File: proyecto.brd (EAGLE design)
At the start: 95.8 x 48.2 mm, 51 parts, among them IC1 ADE9153AACPZ, J1 796638-3, K1 PR28-3V-360-1A-E, Q1 12.288M, Q2 BSS123, U1 ESP32-PICO-MINI-02-N8R2ESP32-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

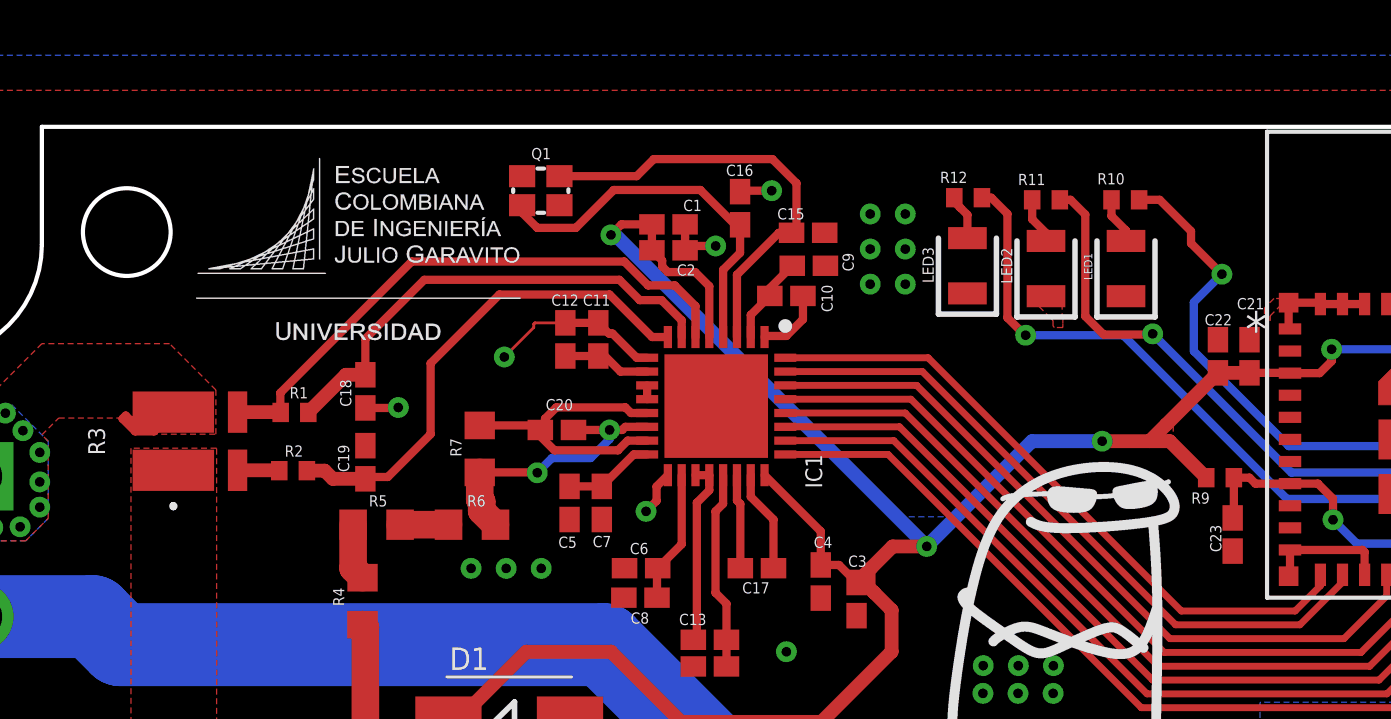
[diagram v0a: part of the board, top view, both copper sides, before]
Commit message: XDIN
XDIN
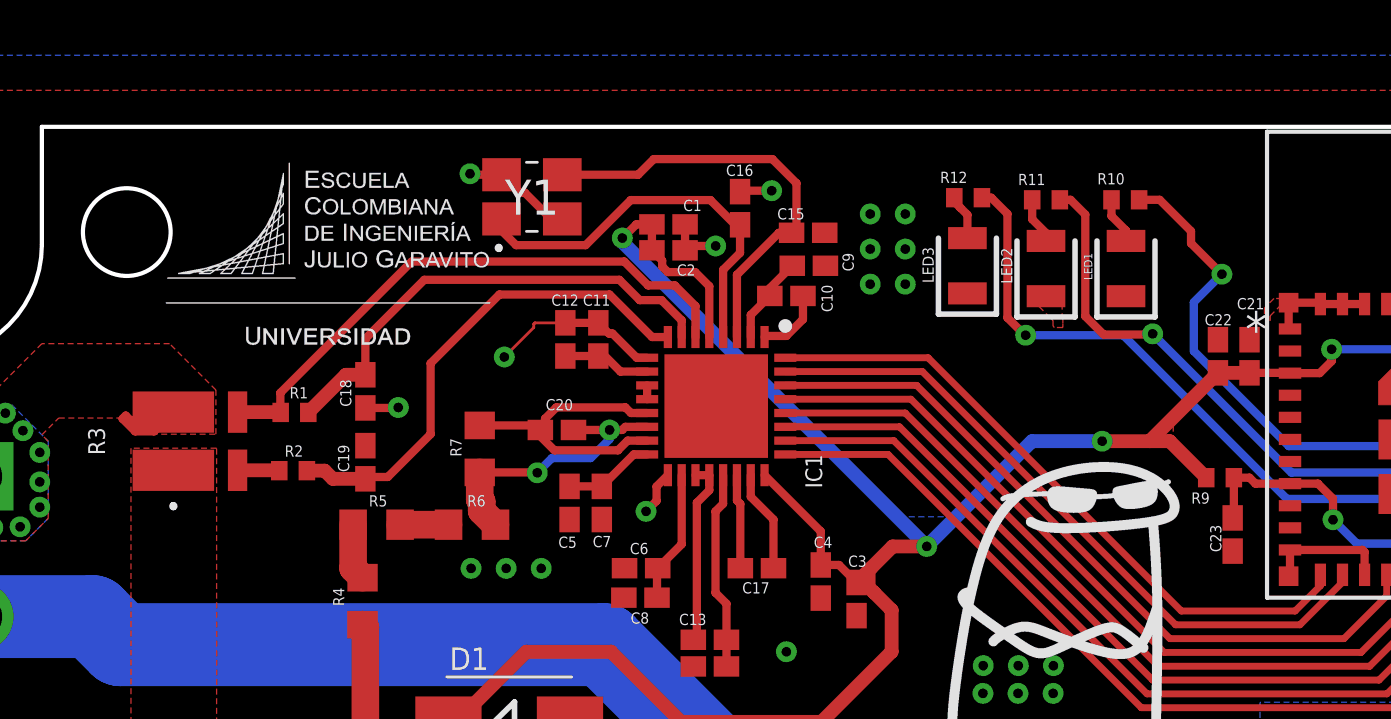
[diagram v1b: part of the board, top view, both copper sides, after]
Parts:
- removed Q1: 12.288M, crystal-geyer_V1_0:2.0X1.6_KX-5
- added Y1: NX3225GA-12.288M-STD-CRG-2, SamacSys_Parts:NX3225GA12288MSTDCRG2
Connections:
- net CLKIN: now also Y1.1; no longer Q1.1
- net CLKOUT: now also Y1.3; no longer Q1.3
- net GND: now also Y1.2, Y1.4
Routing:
- net GND: track 31.8 -> 35.8 mm, vias 45 -> 46
- net CLKIN: track 13.8 -> 14.6 mm
- net +3V3: track 137.3 -> 136.6 mm
